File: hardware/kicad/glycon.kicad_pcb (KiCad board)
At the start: 2 copper layers, 115 x 115 mm, 67 parts, among them IC2 CTC-DIP-28, J1 Conn_02x20_Odd_Even, J2 Conn_01x06, J3 Conn_02x24_Odd_Even, J4 USB_B, Q1 IRF9540N, Q2 IRF9540N, SW1 SW_Push, SW2 SW_Push, U0 Z80CPU, U1 BS62LV1027, U10 74HC244, U11 PIO-DIP-40, U2 SST39SF010, U3 74HC32, U5 74LS08, U6 74LS139, U7 SIO0-DIP-40, U8 PIO-DIP-40, U9 74HC244, X1 ACO-6.144MHz

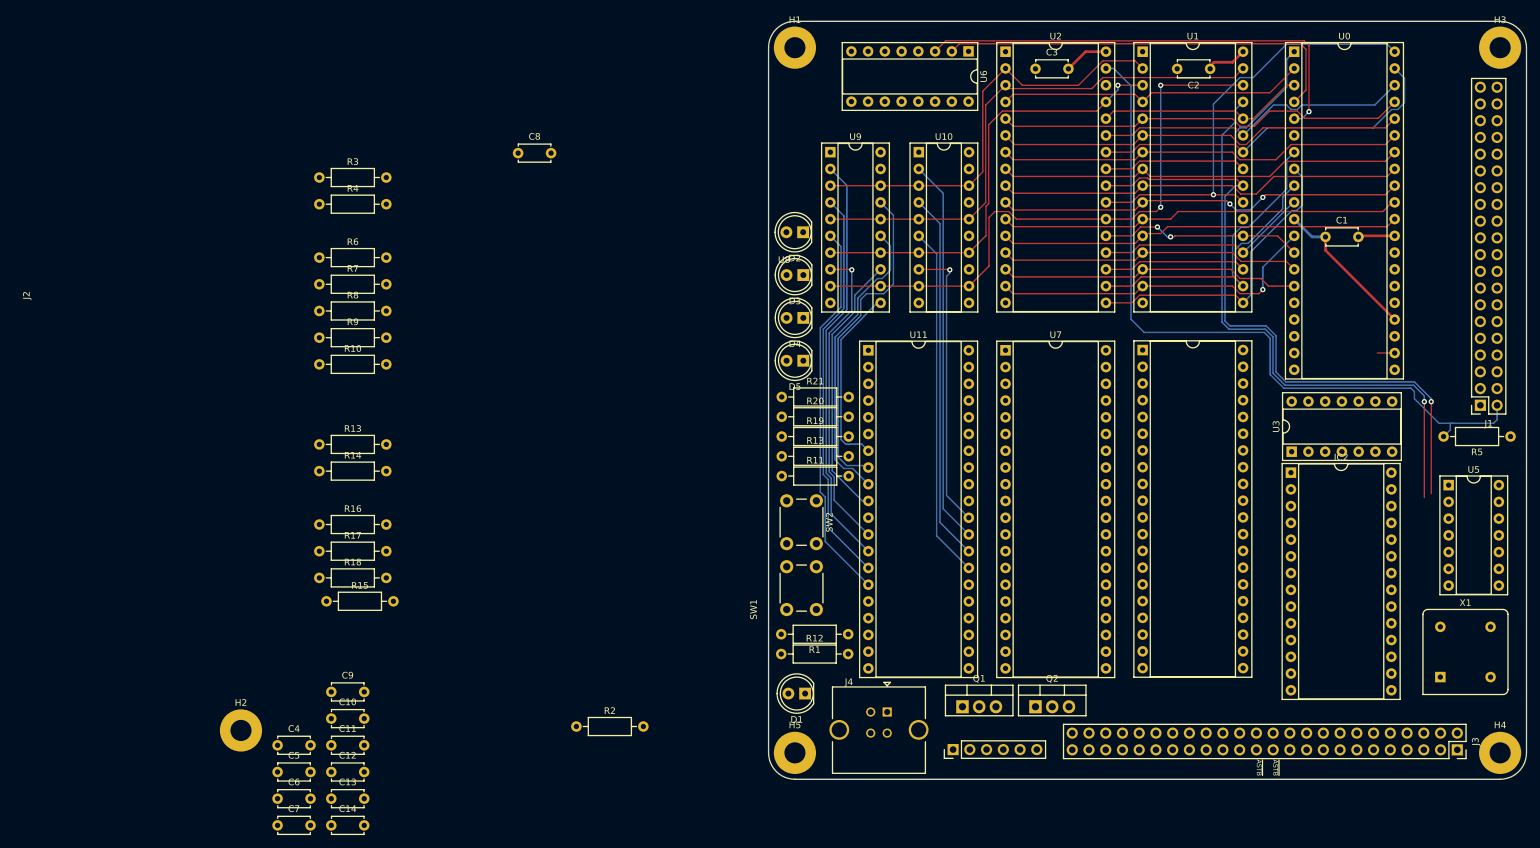
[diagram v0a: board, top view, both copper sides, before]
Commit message: kicad work
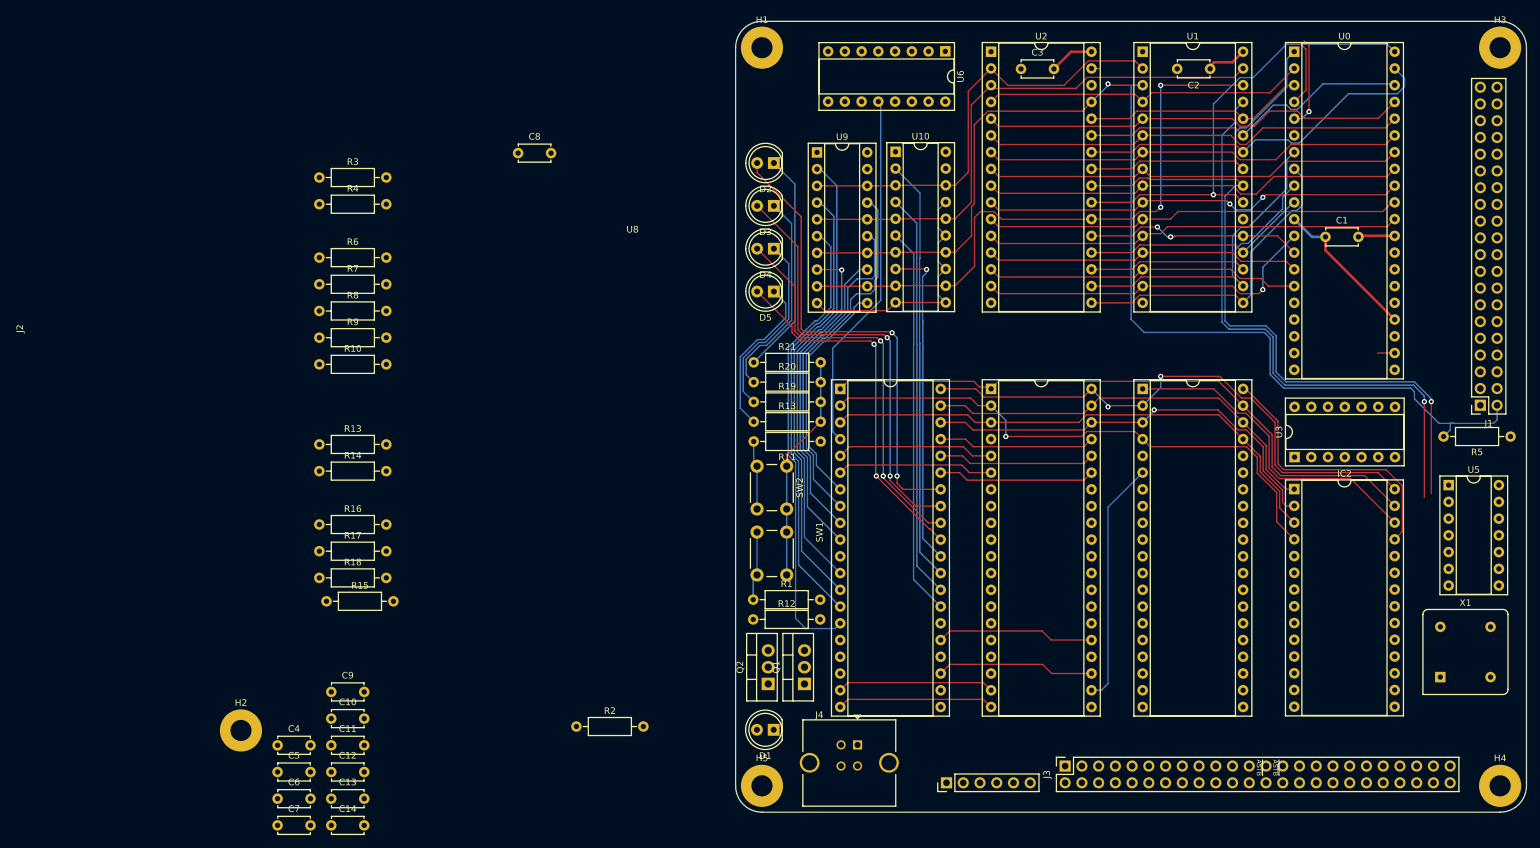
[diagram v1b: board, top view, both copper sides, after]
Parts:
- moved J3 59.6 mm to (201.0, 133.0), turned to 90 degrees
- moved Q2 40.7 mm to (155.9, 120.5), turned to 90 degrees
- moved Q1 24.2 mm to (161.4, 120.5), turned to 90 degrees
- moved U8 23.7 mm to (189.8, 75.8)
- moved U7 21.6 mm to (212.8, 75.8)
- moved R1 15.3 mm to (153.7, 107.8), turned to 0 degrees
- moved SW1 11.8 mm to (158.8, 97.5), turned to -90 degrees
- moved D3 11.4 mm to (156.8, 48.0)
- moved D4 11.4 mm to (156.8, 54.5)
- moved D5 11.4 mm to (156.8, 61.0)
- moved D2 11.4 mm to (156.8, 41.5)
- moved R11 7.91 mm to (163.9, 83.8), turned to 180 degrees
- moved D1 7.28 mm to (156.8, 127.5)
- moved U11 7.25 mm to (166.9, 75.8)
- moved H5 7.07 mm to (155.0, 136.0)
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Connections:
- IC2 pad 11: /IE10 -> /IEI0
- J3 pad 1: +5V -> Earth
- J3 pad 10: /PC2 -> /~{RTSA}
- J3 pad 11: /TO1 -> Earth
- J3 pad 12: /PC1 -> +5V
- J3 pad 13: /CLK -> /PA6
- J3 pad 14: /PC0 -> /PA7
- J3 pad 15: +5V -> /PA4
- J3 pad 16: Earth -> /PA5
- J3 pad 17: /PB6 -> /PA2
- J3 pad 18: /PB7 -> /PA3
- J3 pad 19: /PB4 -> /PA0
- J3 pad 2: Earth -> +5V
- J3 pad 20: /PB5 -> /PA1
- J3 pad 21: /PB2 -> /ARDY
- J3 pad 22: /PB3 -> /~{ASTB}
- J3 pad 23: /PB0 -> /BRDY
- J3 pad 24: /PB1 -> /~{BSTB}
- J3 pad 25: /~{BSTB} -> /PB1
- J3 pad 26: /BRDY -> /PB0
- J3 pad 27: /~{ASTB} -> /PB3
- J3 pad 28: /ARDY -> /PB2
- J3 pad 29: /PA1 -> /PB5
- J3 pad 3: /CT3 -> /RXDA
- J3 pad 30: /PA0 -> /PB4
- J3 pad 31: /PA3 -> /PB7
- J3 pad 32: /PA2 -> /PB6
- J3 pad 33: /PA5 -> Earth
- J3 pad 34: /PA4 -> +5V
- J3 pad 35: /PA7 -> /PC0
- J3 pad 36: /PA6 -> /CLK
- J3 pad 37: +5V -> /PC1
- J3 pad 38: Earth -> /TO1
- J3 pad 39: /~{RTSA} -> /PC2
- J3 pad 4: unconnected-(J3-Pin_4-Pad4) -> /~{DCDA}
- J3 pad 40: /TXDA -> /TO2
- J3 pad 41: /~{CTSA} -> /PC3
- J3 pad 42: /~{W}/~{RDYA} -> /CT1
- J3 pad 43: /~{DTRA} -> /RESET
- J3 pad 44: /SYNCA -> /CT2
- J3 pad 45: /~{DCDA} -> unconnected-(J3-Pin_45-Pad45)
- J3 pad 46: /RXDA -> /CT3
- J3 pad 47: +5V -> Earth
- J3 pad 48: Earth -> +5V
- J3 pad 5: /CT2 -> /SYNCA
- J3 pad 6: /RESET -> /~{DTRA}
- J3 pad 7: /CT1 -> /~{W}/~{RDYA}
- J3 pad 8: /PC3 -> /~{CTSA}
- J3 pad 9: /TO2 -> /TXDA
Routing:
- net /D2: track 50.9 -> 149.3 mm
- net /D3: track 46.7 -> 133.9 mm, vias 0 -> 2
- net /D7: track 30.9 -> 117.3 mm, vias 2 -> 3
- net /D6: track 32.7 -> 114.8 mm
- net /D1: track 45.8 -> 121.3 mm
- net Earth: track 5.57 -> 78.6 mm
- net /PC0: track 0.00 -> 72.1 mm, vias 0 -> 2
- net /D0: track 45.8 -> 114.5 mm
- net /D5: track 39.2 -> 106.1 mm, vias 0 -> 1
- net /PC1: track 0.00 -> 66.6 mm, vias 0 -> 2
- net /D4: track 47.5 -> 112.6 mm
- net /PC2: track 0.00 -> 61.0 mm, vias 0 -> 2
- net /PGA1: track 70.6 -> 13.9 mm
- net /PC3: track 0.00 -> 55.5 mm, vias 0 -> 2
- net /PIO0_~{CE}: track 0.00 -> 54.9 mm
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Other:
- board size 115 x 115 mm -> 120 x 120 mm
